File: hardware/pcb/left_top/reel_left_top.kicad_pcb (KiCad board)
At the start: 2 copper layers, 145.9 x 95.9 mm, 25 parts, among them SW1 choc_plate, SW10 choc_plate, SW11 choc_plate, SW12 choc_plate, SW13 choc_plate, SW14 choc_plate, SW15 choc_plate, SW16 choc_plate, SW17 choc_plate, SW2 choc_plate, SW20 choc_plate, SW21 choc_plate, SW22 choc_plate, SW3 choc_plate, SW4 choc_plate, SW5 choc_plate, SW6 choc_plate, SW7 choc_plate, SW8 choc_plate, SW9 choc_plate

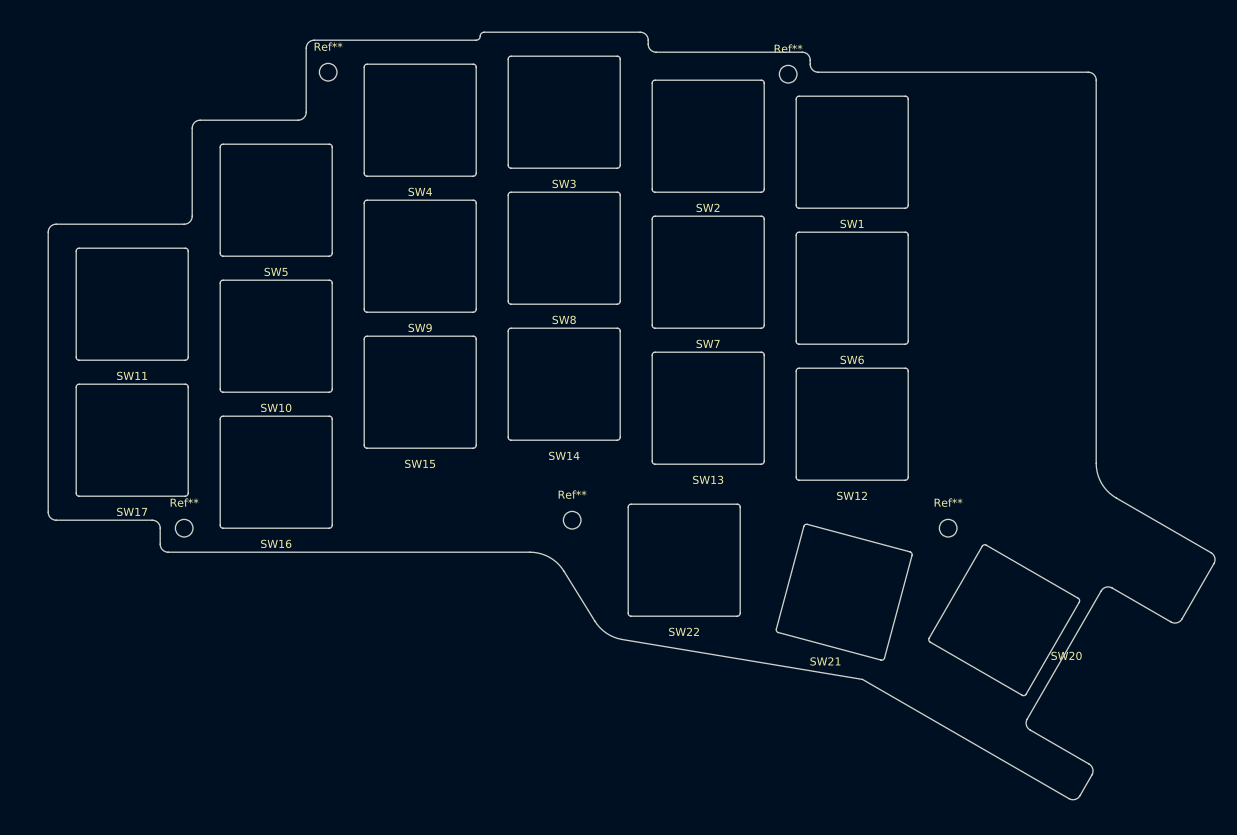
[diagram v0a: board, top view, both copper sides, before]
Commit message: Update ReeL PCB and mechanical assets
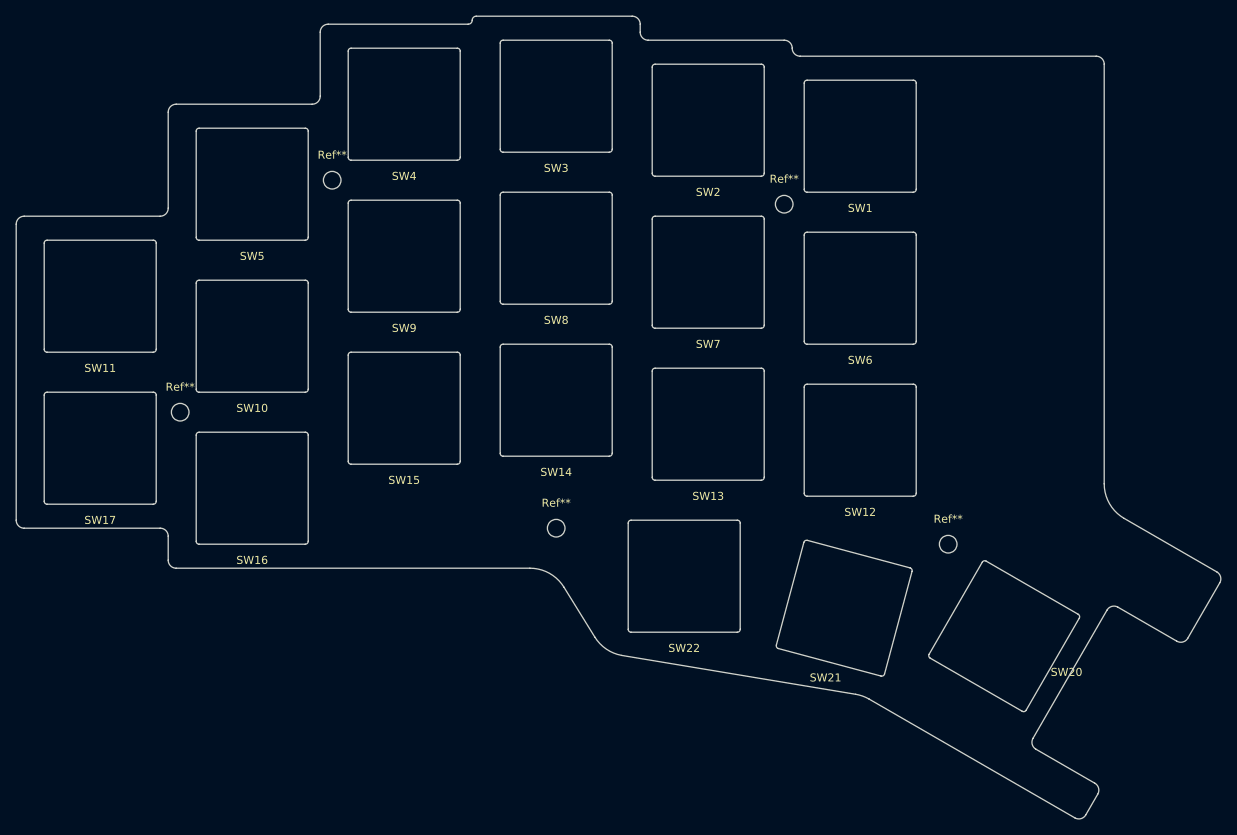
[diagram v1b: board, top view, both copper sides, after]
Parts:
- removed the Ref** at (169.5, 58.2)
- removed the Ref** at (94.0, 115.0)
- removed the Ref** at (112.0, 58.0)
- removed the Ref** at (142.5, 114.0)
- removed the Ref** at (189.5, 115.0)
- added Ref**: MountingHole_2.2mm_M2, MountingHole:MountingHole_2.2mm_M2, F.Cu at (140.5, 115.0)
- added Ref**: MountingHole_2.2mm_M2, MountingHole:MountingHole_2.2mm_M2, F.Cu at (189.5, 117.0)
- added Ref**: MountingHole_2.2mm_M2, MountingHole:MountingHole_2.2mm_M2, F.Cu at (169.0, 74.5)
- added Ref**: MountingHole_2.2mm_M2, MountingHole:MountingHole_2.2mm_M2, F.Cu at (112.5, 71.5)
- added Ref**: MountingHole_2.2mm_M2, MountingHole:MountingHole_2.2mm_M2, F.Cu at (93.5, 100.5)
- moved SW11 4.12 mm to (83.5, 86.0)
- moved SW17 4.12 mm to (83.5, 105.0)
- moved SW16 3.61 mm to (102.5, 110.0)
- moved SW5 3.61 mm to (102.5, 72.0)
- moved SW10 3.00 mm to (102.5, 91.0)
- moved SW15 2.83 mm to (121.5, 100.0)
- moved SW4 2.83 mm to (121.5, 62.0)
- moved SW1 2.24 mm to (178.5, 66.0)
- moved SW12 2.24 mm to (178.5, 104.0)
- moved SW14 2.24 mm to (140.5, 99.0)
- moved SW3 2.24 mm to (140.5, 61.0)
- moved SW13 2.00 mm to (159.5, 102.0)
- moved SW2 2.00 mm to (159.5, 64.0)
- moved SW20 2.00 mm to (196.5, 128.5)
- moved SW21 2.00 mm to (176.5, 125.0)
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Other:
- board size 145.9 x 95.9 mm -> 150.6 x 100.3 mm
